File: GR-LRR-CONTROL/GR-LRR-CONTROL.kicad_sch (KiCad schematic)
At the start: 54 parts, among them IC1 TJA1049T,118, IC2 MC1413DR2G, J1 87833-1019, J10 430451000, J11 87833-1019, J12 10018783-10101TLF, J14 430451000, J15 87833-1019, J16 10018783-10101TLF, J18 691137710002, J2 430451000, J20 901362102, J21 ENC1, J22 ENC2, J23 901362104, J24 LED, J25 UT1, J26 UT2, J3 10018783-10101TLF, J39 Conn_02x12_Counter_Clockwise, J5 DT13-08PB, J6 430451000, J7 87833-1019, J8 10018783-10101TLF, Q1 BSS806NH6327XTSA1, SW1 XA1E-BV302-R, U1 ABX00042, U3 1k

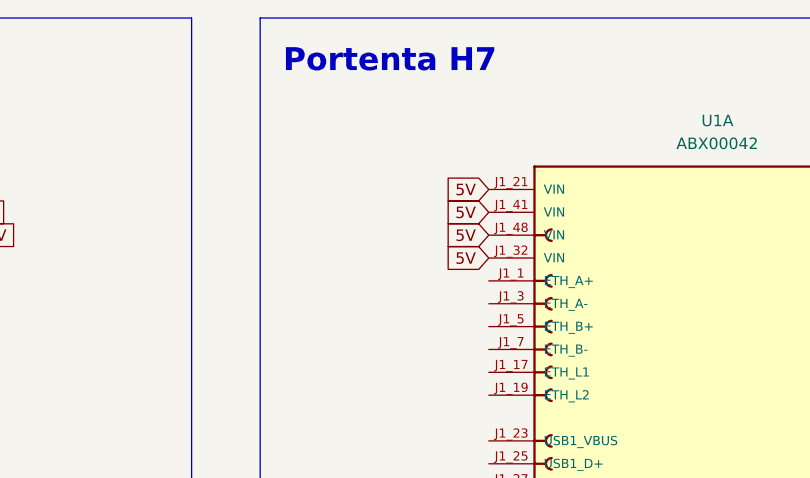
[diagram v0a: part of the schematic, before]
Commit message: ordered power and control A4
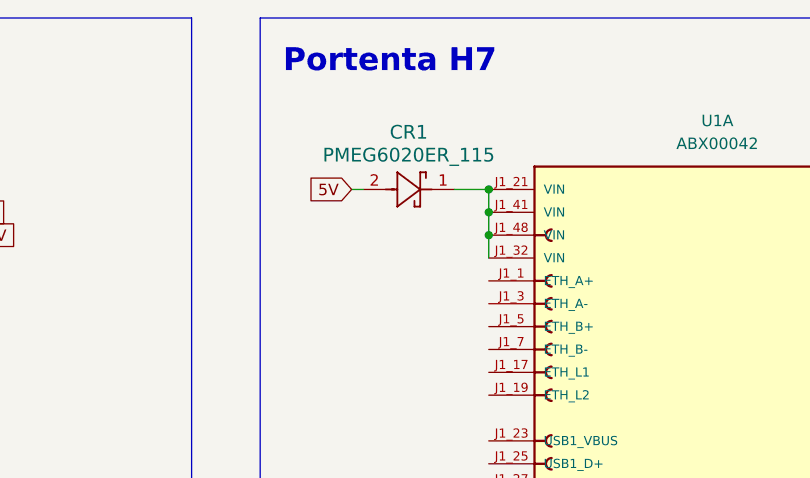
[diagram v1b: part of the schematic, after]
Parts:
- added CR1: PMEG6020ER_115, avid_footprints:CFP3_SOD123W_NEX, symbol avid_symbols:PMEG6020ER_115
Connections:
- net 5V: now also CR1.2; no longer U1.J1_21 (VIN), U1.J1_32 (VIN), U1.J1_41 (VIN), U1.J1_48 (VIN)
- new net: CR1.1, U1.J1_21 (VIN), U1.J1_32 (VIN), U1.J1_41 (VIN), U1.J1_48 (VIN)
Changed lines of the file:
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@@
 	)
 	(junction
+		(at 151.13 44.45)
+		(diameter 0)
+		(color 0 0 0 0)
+	)
+	(junction
 		(at 25.4 317.5)
 		(diameter 0)
@@
 	)
 	(junction
+		(at 151.13 41.91)
+		(diameter 0)
+		(color 0 0 0 0)
+	)
+	(junction
+		(at 151.13 39.37)
+		(diameter 0)
+		(color 0 0 0 0)
+	)
+	(junction
 		(at 450.85 436.88)
 		(diameter 0)
@@
 	(wire
 		(pts
+			(xy 147.32 39.37) (xy 151.13 39.37)
+		)
+		(stroke
+			(width 0)
+			(type default)
+		)
+	)
+	(wire
+		(pts
+			(xy 135.89 39.37) (xy 137.16 39.37)
+		)
+		(stroke
+			(width 0)
+			(type default)
+		)
+	)
+	(wire
+		(pts
 			(xy 590.55 224.79) (xy 622.3 224.79)
 		)
@@
 	(wire
 		(pts
+			(xy 151.13 39.37) (xy 151.13 41.91)
+		)
+		(stroke
+			(width 0)
+			(type default)
+		)
+	)
+	(wire
+		(pts
 			(xy 193.04 226.06) (xy 189.23 226.06)
 		)
@@
 	(wire
 		(pts
+			(xy 151.13 41.91) (xy 151.13 44.45)
+		)
+		(stroke
+			(width 0)
+			(type default)
+		)
+	)
+	(wire
+		(pts
 			(xy 168.91 229.87) (xy 189.23 229.87)
 		)
@@
 	(wire
 		(pts
+			(xy 151.13 44.45) (xy 151.13 46.99)
+		)
+		(stroke
+			(width 0)
+			(type default)
+		)
+	)
+	(wire
+		(pts
 			(xy 582.93 345.44) (xy 599.44 345.44)
 		)
@@
 		)
 	)
+	(global_label "5V"
+		(shape input)
+		(at 135.89 39.37 180)
+		(fields_autoplaced yes)
+		(effects
+			(font
+				(size 1.27 1.27)
+			)
+			(justify right)
+		)
+		(property "Intersheetrefs" "${INTERSHEET_REFS}"
+			(at 130.6067 39.37 0)
+			(effects
+				(font
+					(size 1.27 1.27)
+				)
+				(justify right)
+				(hide yes)
+			)
+		)
+	)
 	(global_label "GND"
 		(shape input)
@@
 		)
 	)
-	(global_label "5V"
-		(shape input)
-		(at 151.13 44.45 180)
-		(fields_autoplaced yes)
-		(effects
-			(font
-				(size 1.27 1.27)
-			)
-			(justify right)
-		)
-		(property "Intersheetrefs" "${INTERSHEET_REFS}"
-			(at 145.8467 44.45 0)
-			(effects
-				(font
-					(size 1.27 1.27)
-				)
-				(justify right)
-				(hide yes)
-			)
-		)
-	)
 	(global_label "D4_B+"
 		(shape input)
@@
 		)
 	)
-	(global_label "5V"
-		(shape input)
-		(at 151.13 46.99 180)
-		(fields_autoplaced yes)
-		(effects
-			(font
-				(size 1.27 1.27)
-			)
-			(justify right)
-		)
-		(property "Intersheetrefs" "${INTERSHEET_REFS}"
-			(at 145.8467 46.99 0)
-			(effects
-				(font
-					(size 1.27 1.27)
-				)
-				(justify right)
-				(hide yes)
-			)
-		)
-	)
 	(global_label "D3_HALL1"
 		(shape input)
@@
 		)
 	)
-	(global_label "5V"
-		(shape input)
-		(at 151.13 39.37 180)
-		(fields_autoplaced yes)
-		(effects
-			(font
-				(size 1.27 1.27)
-			)
-			(justify right)
-		)
-		(property "Intersheetrefs" "${INTERSHEET_REFS}"
-			(at 145.8467 39.37 0)
-			(effects
-				(font
-					(size 1.27 1.27)
-				)
-				(justify right)
-				(hide yes)
-			)
-		)
-	)
 	(global_label "D4_+5VOUT"
 		(shape input)
@@
 		)
 	)
-	(global_label "5V"
-		(shape input)
-		(at 151.13 41.91 180)
-		(fields_autoplaced yes)
-		(effects
-			(font
-				(size 1.27 1.27)
-			)
-			(justify right)
-		)
-		(property "Intersheetrefs" "${INTERSHEET_REFS}"
-			(at 145.8467 41.91 0)
-			(effects
-				(font
-					(size 1.27 1.27)
-				)
-				(justify right)
-				(hide yes)
-			)
-		)
-	)
 	(global_label "DVR_OUT0_4"
 		(shape input)
@@
 					(unit 1)
 				)
+			)
+		)
+	)
+	(symbol
+		(lib_id "avid_symbols:PMEG6020ER_115")
+		(at 137.16 39.37 0)
+		(unit 1)
+		(exclude_from_sim no)
+		(in_bom yes)
+		(on_board yes)
+		(dnp no)
+		(fields_autoplaced yes)
+		(property "Reference" "CR1"
+			(at 142.24 33.02 0)
+			(effects
+				(font
+					(size 1.524 1.524)
+				)
+			)
+		)
+		(property "Value" "PMEG6020ER_115"
+			(at 142.24 35.56 0)
+			(effects
+				(font
+					(size 1.524 1.524)
+				)
+			)
+		)
+		(property "Footprint" "avid_footprints:CFP3_SOD123W_NEX"
+			(at 137.16 39.37 0)
+			(effects
+				(font
+					(size 1.27 1.27)
+					(italic yes)
+				)
+				(hide yes)
+			)
+		)
+		(property "Datasheet" "PMEG6020ER_115"
+			(at 137.16 39.37 0)
+			(effects
+				(font
+					(size 1.27 1.27)
+					(italic yes)
+				)
+				(hide yes)
+			)
+		)
+		(property "Description" ""
+			(at 137.16 39.37 0)
+			(effects
+				(font
+					(size 1.27 1.27)
+				)
+				(hide yes)
+			)
+		)
+		(pin "1"
+		)
+		(pin "2"
+		)
+		(instances
+			(project "GR-LRR-CONTROL"
+				(path "/7e750e3c-c787-4adb-8081-69356fc148e5"
+					(reference "CR1")
+					(unit 1)
+				)
